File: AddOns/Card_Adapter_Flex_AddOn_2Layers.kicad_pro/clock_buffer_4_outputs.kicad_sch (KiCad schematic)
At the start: 12 parts, among them U1 5PB1214

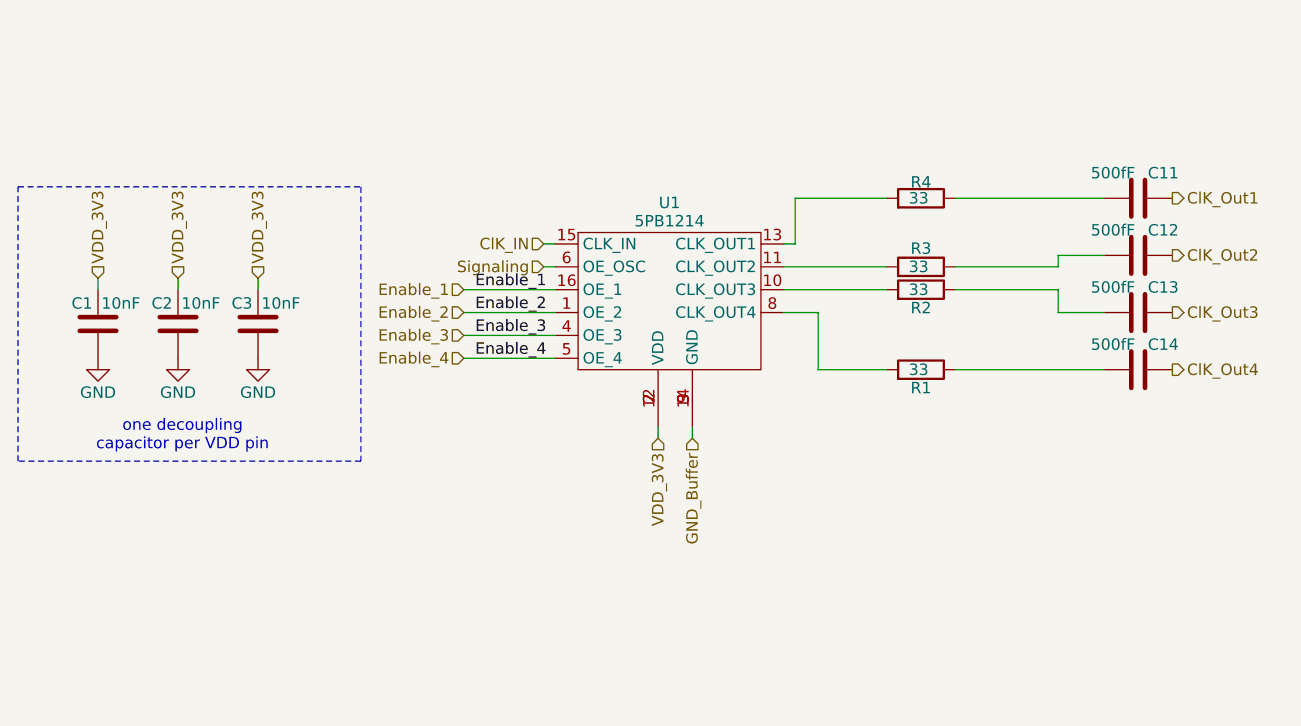
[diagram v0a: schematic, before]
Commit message: .
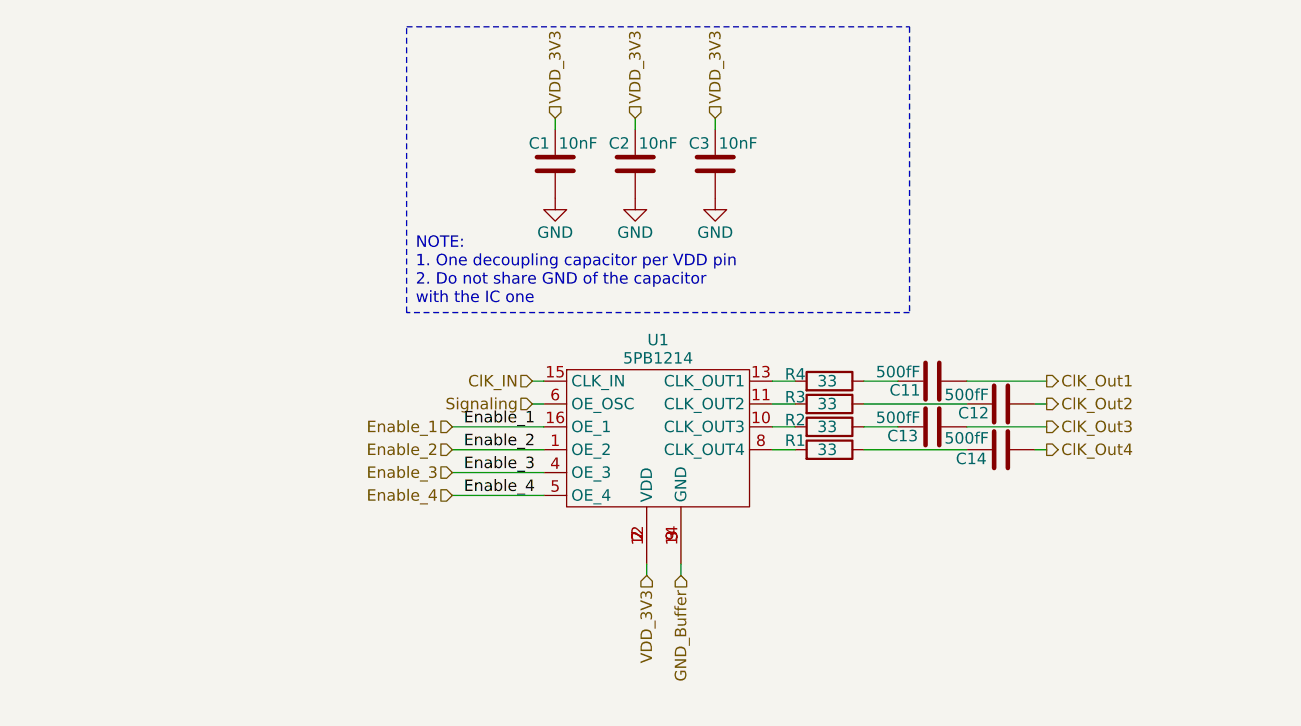
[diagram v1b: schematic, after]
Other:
- note added: "NOTE: 1. One decoupling capacitor per VDD pin 2. Do not share GND of the capacitor with the IC one"
- note removed: "one decoupling capacitor per VDD pin"
- moved on the sheet: C1, C11, C12, C13, C14, C2, C3, R1, R2, R3, R4, U1
